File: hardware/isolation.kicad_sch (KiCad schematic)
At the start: 14 parts, among them IC2 UCC12040DVER, IC3 MCP1700T-3302E_TT, IC4 ISO7742DBQR, IC5 ISO7741DBQR

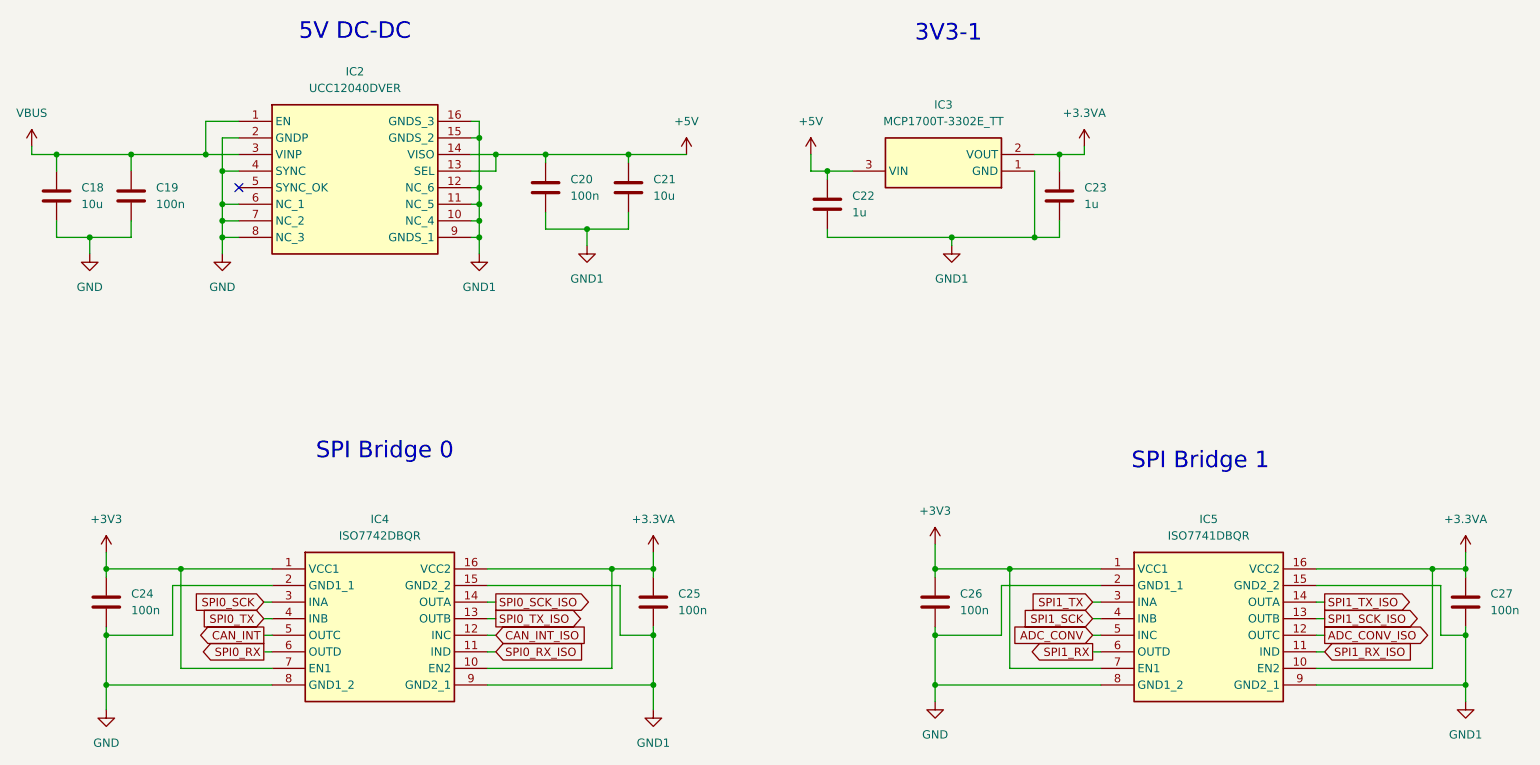
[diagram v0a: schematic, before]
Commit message: Further iso bridge development
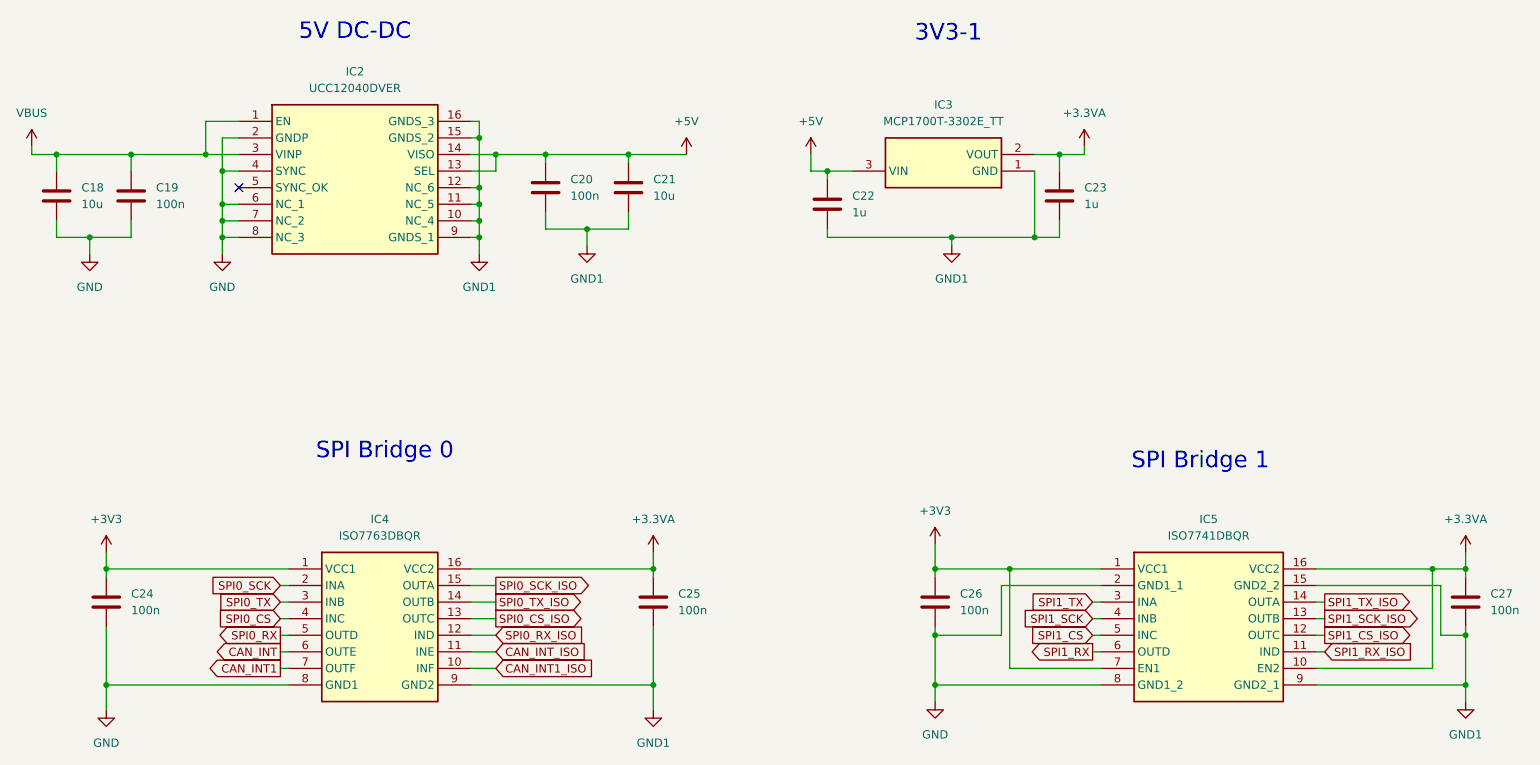
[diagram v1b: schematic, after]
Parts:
- removed IC4: ISO7742DBQR, Stuttgart:SOP64P600X175-16N, symbol Stuttgart:ISO7742DBQR
- added IC4: ISO7763DBQR, Stuttgart:SOP64P600X175-16N, symbol Stuttgart:ISO7763DBQR
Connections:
- net +3.3VA: now also IC4.16 (VCC2)
- net +3V3: now also IC4.1 (VCC1)
- net CAN_INT: now also IC4.6 (OUTE)
- net CAN_INT_ISO: now also IC4.11 (INE)
- net GND: now also IC4.8 (GND1)
- net GND1: now also IC4.9 (GND2)
- net SPI0_RX: now also IC4.5 (OUTD)
- net SPI0_RX_ISO: now also IC4.12 (IND)
- net SPI0_SCK: now also IC4.2 (INA)
- net SPI0_SCK_ISO: now also IC4.15 (OUTA)
- net SPI0_TX: now also IC4.3 (INB)
- net SPI0_TX_ISO: now also IC4.14 (OUTB)
- net ADC_CONV renamed SPI1_CS
- net ADC_CONV_ISO renamed SPI1_CS_ISO
- new net CAN_INT1: IC4.7 (OUTF)
- new net CAN_INT1_ISO: IC4.10 (INF)
- new net SPI0_CS: IC4.4 (INC)
- new net SPI0_CS_ISO: IC4.13 (OUTC)
